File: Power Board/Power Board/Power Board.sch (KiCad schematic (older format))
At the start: 9 parts

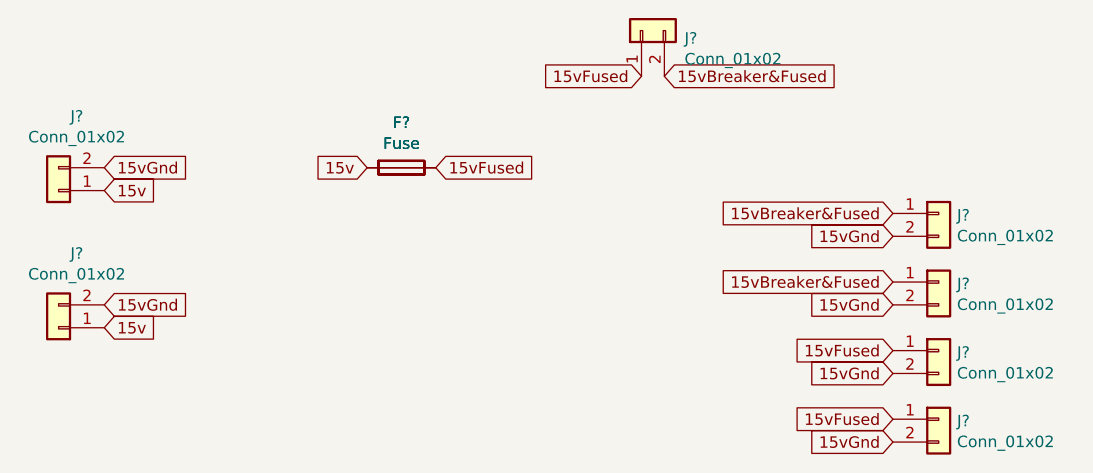
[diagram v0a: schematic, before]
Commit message: final
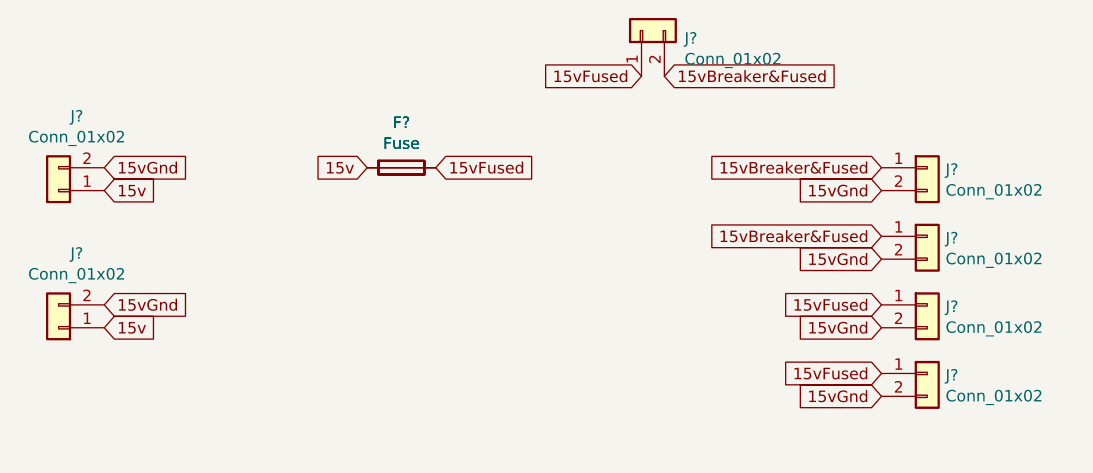
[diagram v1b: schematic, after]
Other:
- moved on the sheet: J?
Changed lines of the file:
@@
 L Connector_Generic:Conn_01x02 J?
 U 1 1 5DA3B29F
-P 5800 3100
-F 0 "J?" H 5880 3092 50  0000 L CNN
-F 1 "Conn_01x02" H 5880 3001 50  0000 L CNN
-F 2 "" H 5800 3100 50  0001 C CNN
-F 3 "~" H 5800 3100 50  0001 C CNN
-	1    5800 3100
+P 5750 2900
+F 0 "J?" H 5830 2892 50  0000 L CNN
+F 1 "Conn_01x02" H 5830 2801 50  0000 L CNN
+F 2 "" H 5750 2900 50  0001 C CNN
+F 3 "~" H 5750 2900 50  0001 C CNN
+	1    5750 2900
 	1    0    0    -1
 $EndComp
@@
 L Connector_Generic:Conn_01x02 J?
 U 1 1 5DA3B2F3
-P 5800 2800
-F 0 "J?" H 5880 2792 50  0000 L CNN
-F 1 "Conn_01x02" H 5880 2701 50  0000 L CNN
-F 2 "" H 5800 2800 50  0001 C CNN
-F 3 "~" H 5800 2800 50  0001 C CNN
-	1    5800 2800
+P 5750 2600
+F 0 "J?" H 5830 2592 50  0000 L CNN
+F 1 "Conn_01x02" H 5830 2501 50  0000 L CNN
+F 2 "" H 5750 2600 50  0001 C CNN
+F 3 "~" H 5750 2600 50  0001 C CNN
+	1    5750 2600
 	1    0    0    -1
 $EndComp
@@
 L Connector_Generic:Conn_01x02 J?
 U 1 1 5DA3B3BF
-P 5800 2500
-F 0 "J?" H 5880 2492 50  0000 L CNN
-F 1 "Conn_01x02" H 5880 2401 50  0000 L CNN
-F 2 "" H 5800 2500 50  0001 C CNN
-F 3 "~" H 5800 2500 50  0001 C CNN
-	1    5800 2500
+P 5750 2300
+F 0 "J?" H 5830 2292 50  0000 L CNN
+F 1 "Conn_01x02" H 5830 2201 50  0000 L CNN
+F 2 "" H 5750 2300 50  0001 C CNN
+F 3 "~" H 5750 2300 50  0001 C CNN
+	1    5750 2300
 	1    0    0    -1
 $EndComp
@@
 L Connector_Generic:Conn_01x02 J?
 U 1 1 5DA3B411
-P 5800 2200
-F 0 "J?" H 5880 2192 50  0000 L CNN
-F 1 "Conn_01x02" H 5880 2101 50  0000 L CNN
-F 2 "" H 5800 2200 50  0001 C CNN
-F 3 "~" H 5800 2200 50  0001 C CNN
-	1    5800 2200
+P 5750 2000
+F 0 "J?" H 5830 1992 50  0000 L CNN
+F 1 "Conn_01x02" H 5830 1901 50  0000 L CNN
+F 2 "" H 5750 2000 50  0001 C CNN
+F 3 "~" H 5750 2000 50  0001 C CNN
+	1    5750 2000
 	1    0    0    -1
 $EndComp
-Text GLabel 5600 3200 0    50   Input ~ 0
+Text GLabel 5550 3000 0    50   Input ~ 0
 15vGnd
-Text GLabel 5600 2900 0    50   Input ~ 0
+Text GLabel 5550 2700 0    50   Input ~ 0
 15vGnd
-Text GLabel 5600 2600 0    50   Input ~ 0
+Text GLabel 5550 2400 0    50   Input ~ 0
 15vGnd
-Text GLabel 5600 2300 0    50   Input ~ 0
+Text GLabel 5550 2100 0    50   Input ~ 0
 15vGnd
-Text GLabel 5600 3100 0    50   Input ~ 0
+Text GLabel 5550 2900 0    50   Input ~ 0
 15vFused
-Text GLabel 5600 2800 0    50   Input ~ 0
+Text GLabel 5550 2600 0    50   Input ~ 0
 15vFused
 $Comp
@@
 Text GLabel 4600 1600 2    50   Input ~ 0
 15vBreaker&Fused
-Text GLabel 5600 2200 0    50   Input ~ 0
+Text GLabel 5550 2000 0    50   Input ~ 0
 15vBreaker&Fused
-Text GLabel 5600 2500 0    50   Input ~ 0
+Text GLabel 5550 2300 0    50   Input ~ 0
 15vBreaker&Fused
 $EndSCHEMATC
